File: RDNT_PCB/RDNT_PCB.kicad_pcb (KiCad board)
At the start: 2 copper layers, 118.9 x 77.6 mm, 41 parts, among them IC1 TPS563300DRLR, J1 AudioJack3, J2 AudioJack3, J3 Conn_02x05_Counter_Clockwise, SW1 SW_MEC_5E, U1 TMUX1309QDYYRQ1, U2 ESP32-WROOM-32, U6 LM324

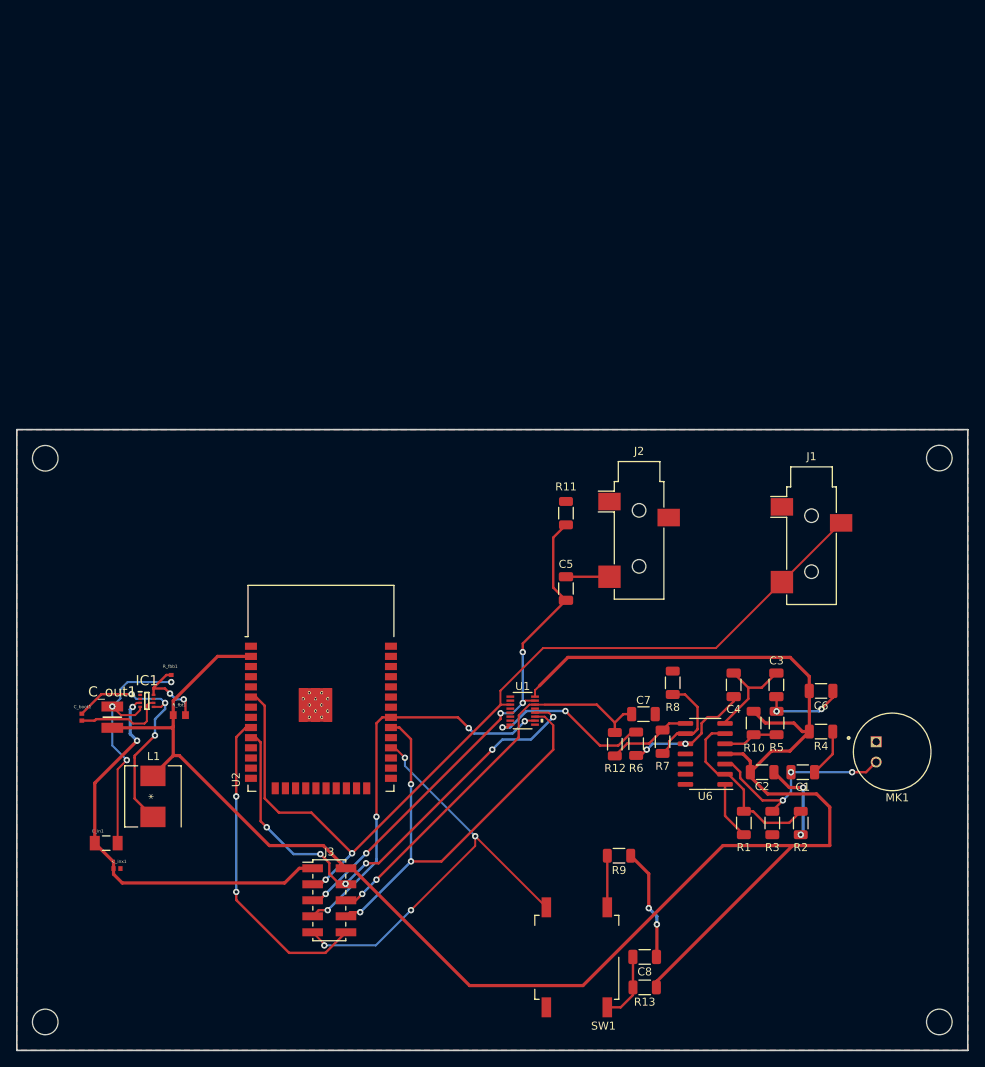
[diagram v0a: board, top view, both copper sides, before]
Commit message: PCB Updated
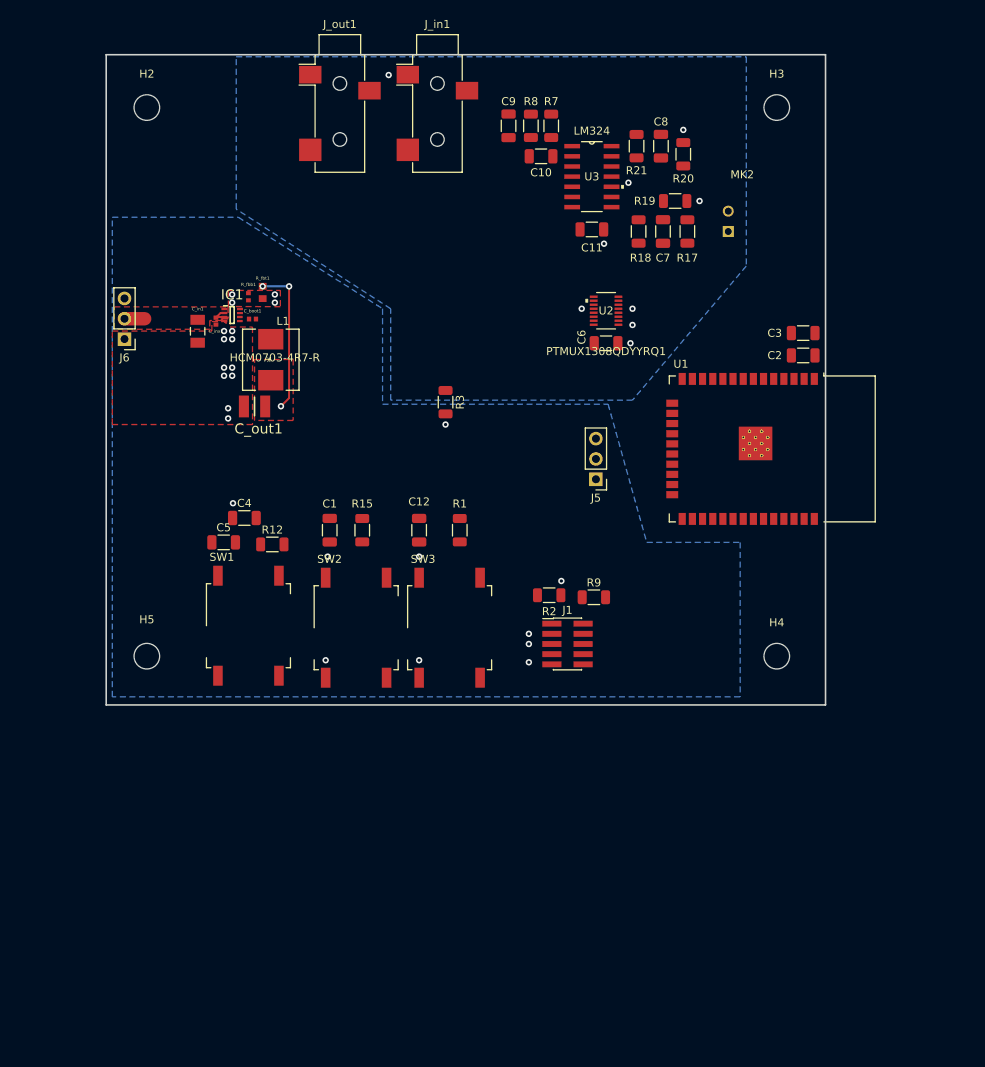
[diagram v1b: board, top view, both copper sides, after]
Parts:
- removed H1: MountingHole, MountingHole:MountingHole_3.2mm_M3
- removed J2: AudioJack3, Connector_Audio:Jack_3.5mm_CUI_SJ-3523-SMT_Horizontal
- removed J3: Conn_02x05_Counter_Clockwise, Connector_PinHeader_2.00mm:PinHeader_2x05_P2.00mm_Vertical_SMD
- removed MK1: CMA-4544PF-W, electret_mic:MIC_CMA-4544PF-W
- removed R10: 68K, Resistor_SMD:R_1206_3216Metric
- removed R11: 330, Resistor_SMD:R_1206_3216Metric
- removed R13, R5: 1K, Resistor_SMD:R_1206_3216Metric
- removed R4: 22K, Resistor_SMD:R_1206_3216Metric
- removed R6: 87, Resistor_SMD:R_1206_3216Metric
- removed U6: LM324, Package_SO:SOIC-14_3.9x8.7mm_P1.27mm
- added C10: 10uF, Capacitor_SMD:C_1206_3216Metric, F.Cu at (135.6, 31.5)
- added C11: 0.1uF, Capacitor_SMD:C_1206_3216Metric, F.Cu at (142.0, 40.6)
- added C12: 0.1uF, Capacitor_SMD:C_1206_3216Metric, F.Cu at (120.4, 78.2)
- added C9: 10uF, Capacitor_SMD:C_1206_3216Metric, F.Cu at (131.6, 27.7)
- added H5: MountingHole, MountingHole:MountingHole_3.2mm_M3, F.Cu at (86.4, 94.0)
- added J5: Screw_Terminal_01x03, Connector_PinHeader_2.54mm:PinHeader_1x03_P2.54mm_Vertical, F.Cu at (142.5, 71.9)
- added J6: Screw_Terminal_01x03, Connector_PinHeader_2.54mm:PinHeader_1x03_P2.54mm_Vertical, F.Cu at (83.6, 54.3)
- added J_in1: AudioJack3, Connector_Audio:Jack_3.5mm_CUI_SJ-3523-SMT_Horizontal, F.Cu at (122.7, 24.9)
- added J_out1: AudioJack3, Connector_Audio:Jack_3.5mm_CUI_SJ-3523-SMT_Horizontal, F.Cu at (110.5, 24.9)
- added MK2: CMA-4544PF-W, electret_mic:MIC_CMA-4544PF-W, B.Cu at (161.0, 39.6)
- added R15: 10K, Resistor_SMD:R_1206_3216Metric, F.Cu at (113.3, 78.2)
- added R17: 2200, Resistor_SMD:R_1206_3216Metric, F.Cu at (153.9, 40.9)
- added R18: 400000, Resistor_SMD:R_1206_3216Metric, F.Cu at (147.8, 40.9)
- added R19: 100000, Resistor_SMD:R_1206_3216Metric, F.Cu at (152.4, 37.1)
- added R20: 1000, Resistor_SMD:R_1206_3216Metric, F.Cu at (153.4, 31.2)
- added R21: 1500, Resistor_SMD:R_1206_3216Metric, F.Cu at (147.6, 30.2)
- added SW2: SW_MEC_5E, Button_Switch_SMD:SW_MEC_5GSH9, F.Cu at (112.5, 90.4)
- added SW3: SW_MEC_5E, Button_Switch_SMD:SW_MEC_5GSH9, F.Cu at (124.2, 90.4)
- added U3: LM324, Lm324:LM324D, F.Cu at (142.0, 34.0)
- C1: value 1uF -> 0.1uF
- C2: value 470uF -> 0.1uF
- C3: value 100uF -> 10uF
- C4: value 10uF -> 0.1uF
- C5: value 100uF -> 0.1uF
- C7: value 0.1uF -> 1uF
- C8: value .1uF -> 0.033uF
- J1: value AudioJack3 -> Conn_ARM_JTAG_SWD_10; footprint Connector_Audio:Jack_3.5mm_CUI_SJ-3523-SMT_Horizontal -> Connector_PinHeader_1.27mm:PinHeader_2x05_P1.27mm_Vertical_SMD
- R1: value 100K -> 10K
- R12: value 510 -> 1K
- R2, R9: value 1K -> 10K
- R3: value 100K -> 1
- R7: value 390 -> 203K
- R8: value 110 -> 100K
- U1: value TMUX1309QDYYRQ1 -> ESP32-WROOM-32D; footprint TMUX1309QDYYRQ1:TMUX1309QDYYRQ1 -> RF_Module:ESP32-WROOM-32
- U2: value ESP32-WROOM-32 -> PTMUX1308QDYYRQ1; footprint RF_Module:ESP32-WROOM-32 -> TMUX1309QDYYRQ1:PTMUX1308QDYYRQ1
- moved H3 116.1 mm to (165.1, 25.4)
- moved H2 115.0 mm to (86.4, 25.4)
- moved C8 101.4 mm to (150.6, 30.2), turned to 90 degrees
- moved R7 78.2 mm to (136.9, 27.7)
- moved R8 71.8 mm to (134.4, 27.7)
- moved C_inx1 69.5 mm to (95.0, 52.1), turned to -90 degrees
- moved R3 66.6 mm to (123.7, 62.2), turned to -90 degrees
- moved C1 66.4 mm to (109.2, 78.2), turned to -90 degrees
- moved C_in1 65.0 mm to (92.7, 53.4), turned to -90 degrees
- moved C4 64.6 mm to (98.6, 76.7), turned to 0 degrees
- moved U2 61.6 mm to (143.8, 50.8), turned to 180 degrees
- moved C7 60.4 mm to (150.9, 40.9), turned to 90 degrees
- moved SW1 58.3 mm to (99.1, 90.2), turned to 0 degrees
- moved L1 56.5 mm to (101.9, 56.9), turned to 90 degrees
- moved C_boot1 54.1 mm to (99.6, 51.8), turned to 0 degrees
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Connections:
- C1 pad 1: Net-(C1-Pad1) -> /reset
- C1 pad 2: Net-(C1-Pad2) -> DGND
- C2 pad 1: VCC -> DGND
- C2 pad 2: GNDREF -> VCC
- C3 pad 1: Net-(C3-Pad1) -> DGND
- C3 pad 2: GNDREF -> VCC
- C4 pad 1: Net-(C3-Pad1) -> DGND
- C4 pad 2: Net-(C4-Pad2) -> /mode
- C5 pad 1: /Aux_ADC -> VCC
- C6 pad 1: GNDREF -> AGND
- C6 pad 2: VCC -> 5V
- C7 pad 1: /Mic_ADC -> Net-(C7-Pad1)
- C7 pad 2: GNDREF -> Net-(C7-Pad2)
- C8 pad 1: GNDREF -> Net-(C8-Pad1)
- C8 pad 2: Net-(C8-Pad2) -> /Mic_out
- C_in1 pad 1: /+5V -> 5V
- C_in1 pad 2: GNDREF -> DGND
- C_inx1 pad 1: /+5V -> 5V
- C_inx1 pad 2: GNDREF -> DGND
- C_out1 pad 2: GNDREF -> DGND
- IC1 pad 2: unconnected-(IC1-Pad2) -> 5V
- IC1 pad 3: /+5V -> 5V
- IC1 pad 4: GNDREF -> DGND
- R1 pad 1: Net-(R1-Pad1) -> VCC
- R1 pad 2: Net-(R1-Pad2) -> /boot
- R12 pad 1: Net-(R12-Pad1) -> Net-(C5-Pad2)
- R12 pad 2: /Mic_ADC -> /mode
- R2 pad 1: GNDREF -> VCC
- R2 pad 2: Net-(R1-Pad2) -> DGND
- R3 pad 1: GNDREF -> AGND
- R3 pad 2: Net-(C1-Pad2) -> DGND
- R7 pad 1: Net-(R12-Pad1) -> 5V
- R8 pad 2: GNDREF -> AGND
- R9 pad 1: GNDREF -> VCC
- R9 pad 2: Net-(R9-Pad2) -> Net-(J1-Pad10)
- R_fbb1 pad 1: GNDREF -> DGND
- SW1 pad 1: Net-(C8-Pad2) -> Net-(C5-Pad2)
- SW1 pad 2: Net-(R9-Pad2) -> Net-(C5-Pad2)
- SW1 pad 3: unconnected-(SW1-Pad3) -> VCC
- SW1 pad 4: /mode -> VCC
- U1 pad 1: unconnected-(U1-Pad1) -> DGND
- U1 pad 10: /sel2 -> /Ble_DAC
- U1 pad 11: /sel1 -> /DAC_backup
- U1 pad 12: /Ble_DAC -> /Mode_sel
- U1 pad 13: unconnected-(U1-Pad13) -> Net-(J1-Pad2)
- U1 pad 14: /Mic_ADC -> Net-(J1-Pad8)
- U1 pad 15: /Aux_ADC -> DGND
- U1 pad 16: VCC -> Net-(J1-Pad4)
- U1 pad 2: unconnected-(U1-Pad2) -> VCC
- U1 pad 3: /Mux_Out -> /reset
- U1 pad 6: unconnected-(U1-Pad6) -> /ADC_In
- U1 pad 7: unconnected-(U1-Pad7) -> /ADC_backup
- U1 pad 8: GNDREF -> /Mode_backup
- U2 pad 1: GNDREF -> AGND
- U2 pad 10: /Ble_DAC -> /sel2
- U2 pad 11: unconnected-(U2-Pad11) -> /sel1
- U2 pad 12: unconnected-(U2-Pad12) -> AGND
- U2 pad 13: unconnected-(U2-Pad13) -> /Mic_out
- U2 pad 14: unconnected-(U2-Pad14) -> /AUX_mono
- U2 pad 15: GNDREF -> /Ble_DAC
- U2 pad 16: unconnected-(U2-Pad16) -> 5V
- U2 pad 2: VCC -> AGND
- U2 pad 3: unconnected-(U2-Pad3) -> /ADC_In
- U2 pad 4: unconnected-(U2-Pad4) -> AGND
- U2 pad 5: unconnected-(U2-Pad5) -> AGND
- U2 pad 6: /Mux_Out -> AGND
- U2 pad 8: unconnected-(U2-Pad8) -> AGND
- U2 pad 9: /LED_Out -> AGND
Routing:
- net VCC: track 239.4 -> 18.7 mm, vias 0 -> 3
- net /Mux_Out: track 114.6 -> 0.00 mm, vias 2 -> 0
- net GNDREF: track 88.3 -> 0.00 mm, vias 11 -> 0
- net /Aux_ADC: track 64.4 -> 0.00 mm, vias 5 -> 0
- net /Ble_DAC: track 63.2 -> 0.00 mm, vias 6 -> 0
- net /sel1: track 58.7 -> 0.00 mm, vias 3 -> 0
- net /mode: track 55.8 -> 0.00 mm, vias 4 -> 0
- net /+5V: track 51.8 -> 0.00 mm, vias 2 -> 0
- net /Mic_ADC: track 50.1 -> 0.00 mm, vias 2 -> 0
- net /sel2: track 49.7 -> 0.00 mm, vias 4 -> 0
- net /LED_Out: track 40.2 -> 0.00 mm, vias 2 -> 0
- net Net-(C_boot1-Pad2): track 30.3 -> 0.00 mm, vias 3 -> 0
- net Net-(C1-Pad2): track 26.6 -> 0.00 mm, vias 3 -> 0
- net Net-(R1-Pad2): track 22.8 -> 0.00 mm
- net Net-(C4-Pad2): track 16.3 -> 0.00 mm, vias 2 -> 0
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- added copper zone on F.Cu, net 5V
- added copper zone on B.Cu, net AGND
- added copper zone on B.Cu, net DGND
- added copper zone on F.Cu, net DGND
- added copper zone on F.Cu, net VCC
- removed copper zone on B.Cu, net GNDREF
- removed copper zone on F.Cu, net GNDREF
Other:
- board size 118.9 x 77.6 mm -> 89.9 x 81.3 mm
